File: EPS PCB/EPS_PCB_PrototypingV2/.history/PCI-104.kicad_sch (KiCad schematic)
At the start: 8 parts, among them J1 Conn_02x26_Row_Letter_First, J2 Conn_02x26_Row_Letter_First, J3 Conn_01x08_Pin, J4 Conn_01x06_Pin

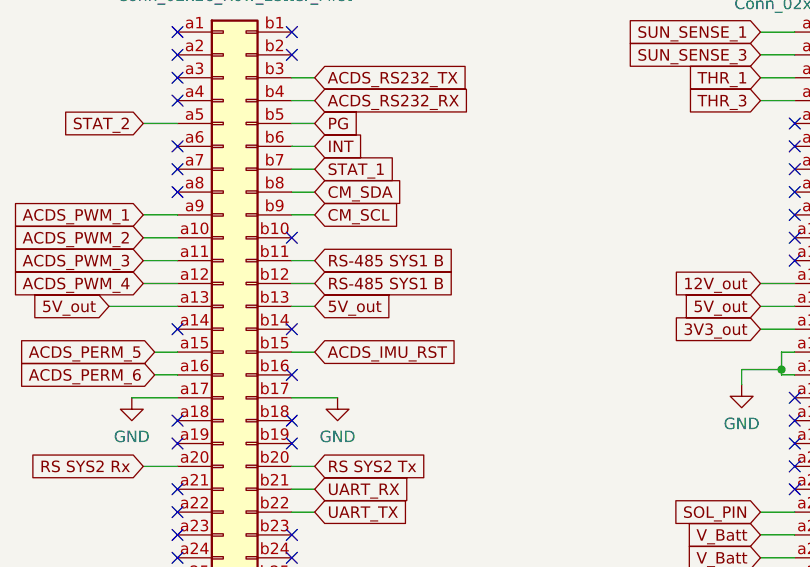
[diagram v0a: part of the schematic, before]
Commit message: Small PC104 Template Fix
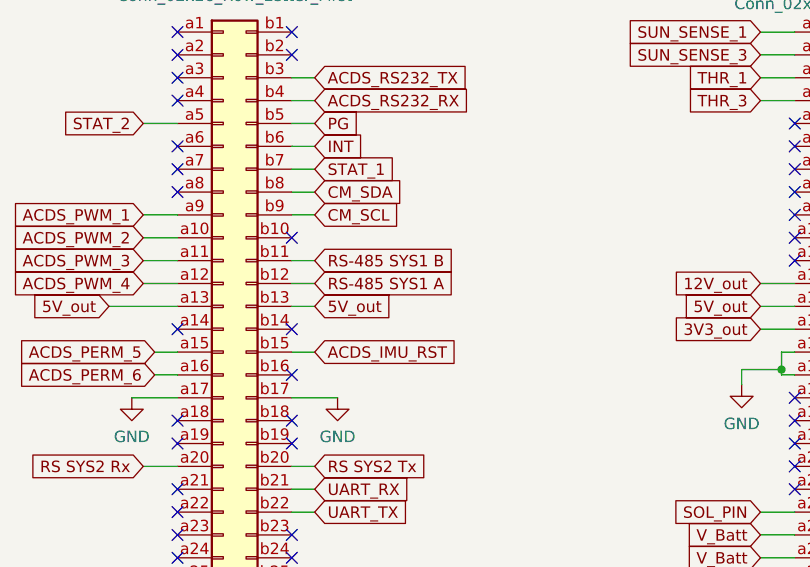
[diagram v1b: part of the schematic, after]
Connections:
- net RS-485 SYS1 B: no longer J1.b12 (Pin_b12)
- new net RS-485 SYS1 A: J1.b12 (Pin_b12)
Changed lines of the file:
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@@
 		)
 	)
-	(global_label "RS-485 SYS1 B"
+	(global_label "RS-485 SYS1 A"
 		(shape input)
 		(at 152.4 83.82 0)
@@
 		)
 		(property "Intersheetrefs" "${INTERSHEET_REFS}"
-			(at 170.9879 83.82 0)
+			(at 170.8065 83.82 0)
 			(hide yes)
 			(show_name no)
